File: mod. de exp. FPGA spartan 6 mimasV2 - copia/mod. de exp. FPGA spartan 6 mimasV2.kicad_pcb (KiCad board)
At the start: 2 copper layers, 111.5 x 57.8 mm, 46 parts, among them J1 locked, J2 locked, J3 locked, J4 locked, SW1 SW_DIP_x08, SW2 SW_Push, SW3 SW_Push, SW4 SW_Push, SW5 SW_Push, U1 CA56-12CGKWA

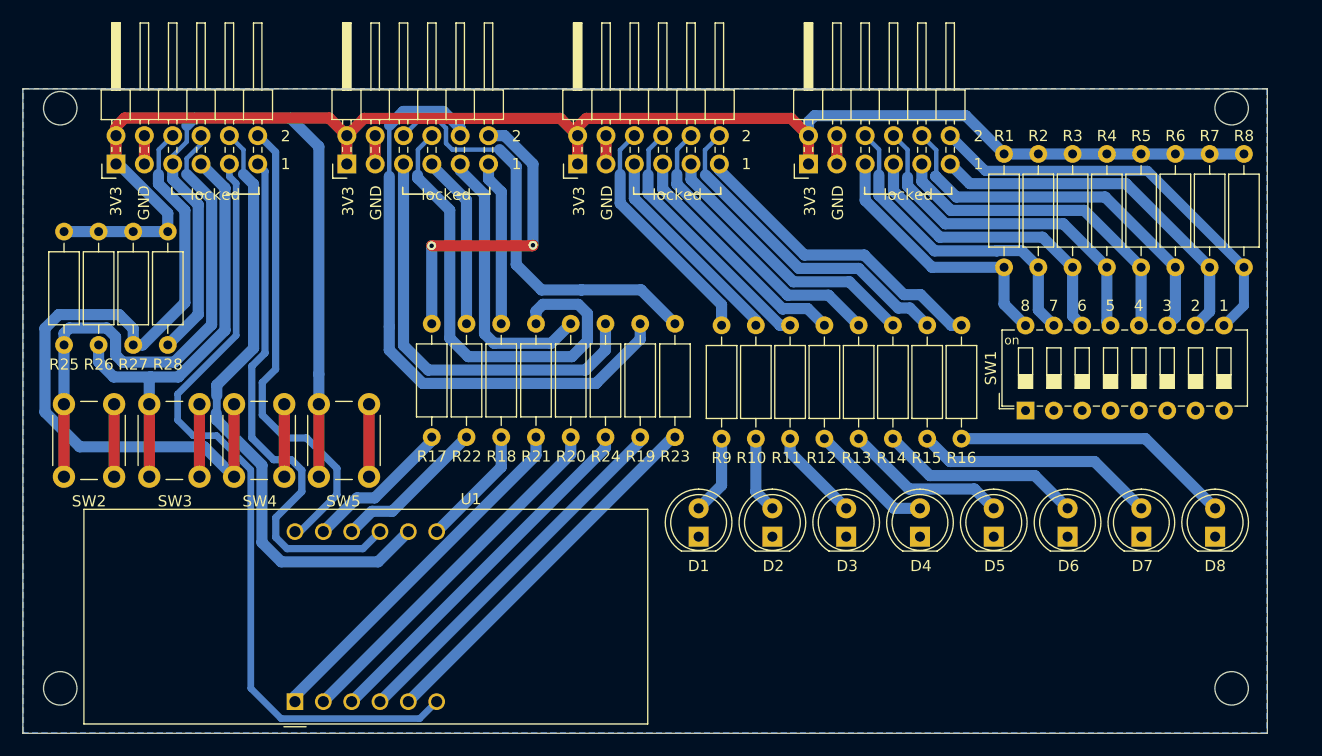
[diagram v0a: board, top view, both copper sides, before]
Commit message: absolutamente todo
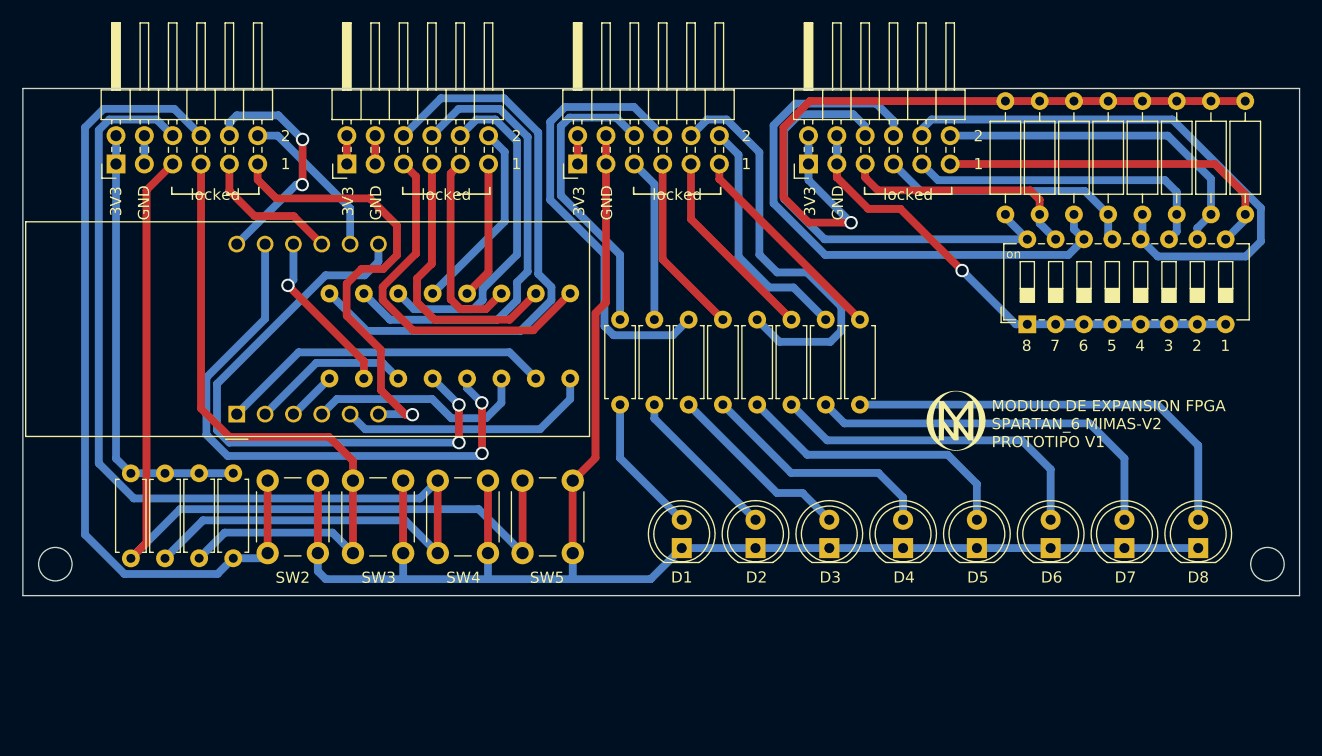
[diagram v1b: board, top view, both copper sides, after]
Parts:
- added G***: LOGO, wao:logo v2, F.Cu at (175.3, 123.0)
- R10, R11, R12, R13, R14, R15, R16, R25, R26, R27, R28, R9: footprint Resistor_THT:R_Axial_DIN0207_L6.3mm_D2.5mm_P10.16mm_Horizontal -> Resistor_THT:R_Axial_DIN0207_L6.3mm_D2.5mm_P7.62mm_Horizontal
- R17, R18, R19, R20, R21, R22, R23, R24: footprint Resistor_THT:R_Axial_DIN0207_L6.3mm_D2.5mm_P10.16mm_Horizontal -> Resistor_THT:R_Axial_DIN0207_L6.3mm_D2.5mm_P7.62mm_Horizontal; moved to B.Cu
- moved R25 26.4 mm to (110.5, 127.7)
- moved U1 26.3 mm to (110.8, 122.4)
- moved R24 24.9 mm to (119.1, 111.6)
- moved R26 23.5 mm to (107.5, 127.7)
- moved R28 21.9 mm to (101.3, 127.7)
- moved R27 21.9 mm to (104.4, 127.7)
- moved SW2 19.5 mm to (118.1, 128.4)
- moved SW4 19.5 mm to (133.3, 128.4)
- moved SW3 19.5 mm to (125.7, 128.4)
- moved SW5 19.5 mm to (140.9, 128.4)
- moved R20 15.7 mm to (125.3, 111.6)
- moved R19 12.7 mm to (134.5, 111.6)
- moved R23 9.77 mm to (140.7, 111.6)
- moved R22 9.59 mm to (122.2, 111.6)
- moved R15 9.11 mm to (163.6, 114.0)
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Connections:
- D1 pad 1: GND -> GND2
- D2 pad 1: GND -> GND2
- D3 pad 1: GND -> GND2
- D4 pad 1: GND -> GND2
- D5 pad 1: GND -> GND2
- D6 pad 1: GND -> GND2
- D7 pad 1: GND -> GND2
- D8 pad 1: GND -> GND2
- J2 pad 1: +3V3 -> +3.3V
- J2 pad 2: +3V3 -> +3.3V
- J2 pad 3: GND -> GND1
- J2 pad 4: GND -> GND1
- J3 pad 1: +3V3 -> +3.3VA
- J3 pad 2: +3V3 -> +3.3VA
- J3 pad 3: GND -> GND2
- J3 pad 4: GND -> GND2
- J4 pad 1: +3V3 -> +3.3VADC
- J4 pad 2: +3V3 -> +3.3VADC
- J4 pad 3: GND -> GND3
- J4 pad 4: GND -> GND3
- R1 pad 1: +3V3 -> +3.3VADC
- R1 pad 2: /DIP_SWITCH/7P9 -> /DIP_SWITCH/8P9
- R17 pad 1: /DISPLAY/2P7 -> /DISPLAY/1P7
- R18 pad 1: /DISPLAY/1P7 -> /DISPLAY/2P7
- R19 pad 1: /DISPLAY/4P7 -> /DISPLAY/3P7
- R2 pad 1: +3V3 -> +3.3VADC
- R2 pad 2: /DIP_SWITCH/8P9 -> /DIP_SWITCH/7P9
- R20 pad 1: /DISPLAY/3P7 -> /DISPLAY/4P7
- R21 pad 1: /DISPLAY/6P7 -> /DISPLAY/5P7
- R22 pad 1: /DISPLAY/5P7 -> /DISPLAY/6P7
- R23 pad 1: /DISPLAY/8P7 -> /DISPLAY/7P7
- R24 pad 1: /DISPLAY/7P7 -> /DISPLAY/8P7
- R3 pad 1: +3V3 -> +3.3VADC
- R3 pad 2: /DIP_SWITCH/5P9 -> /DIP_SWITCH/6P9
- R4 pad 1: +3V3 -> +3.3VADC
- R4 pad 2: /DIP_SWITCH/6P9 -> /DIP_SWITCH/5P9
- R5 pad 1: +3V3 -> +3.3VADC
- R5 pad 2: /DIP_SWITCH/3P9 -> /DIP_SWITCH/4P9
- R6 pad 1: +3V3 -> +3.3VADC
- R6 pad 2: /DIP_SWITCH/4P9 -> /DIP_SWITCH/3P9
- R7 pad 1: +3V3 -> +3.3VADC
- R7 pad 2: /DIP_SWITCH/1P9 -> /DIP_SWITCH/2P9
- R8 pad 1: +3V3 -> +3.3VADC
- R8 pad 2: /DIP_SWITCH/2P9 -> /DIP_SWITCH/1P9
- SW1 pad 1: GND -> GND3
- SW1 pad 10: /DIP_SWITCH/1P9 -> /DIP_SWITCH/2P9
- SW1 pad 11: /DIP_SWITCH/4P9 -> /DIP_SWITCH/3P9
- SW1 pad 12: /DIP_SWITCH/3P9 -> /DIP_SWITCH/4P9
- SW1 pad 13: /DIP_SWITCH/6P9 -> /DIP_SWITCH/5P9
- SW1 pad 14: /DIP_SWITCH/5P9 -> /DIP_SWITCH/6P9
- SW1 pad 15: /DIP_SWITCH/8P9 -> /DIP_SWITCH/7P9
- SW1 pad 16: /DIP_SWITCH/7P9 -> /DIP_SWITCH/8P9
- SW1 pad 2: GND -> GND3
- SW1 pad 3: GND -> GND3
- SW1 pad 4: GND -> GND3
- SW1 pad 5: GND -> GND3
- SW1 pad 6: GND -> GND3
- SW1 pad 7: GND -> GND3
- SW1 pad 8: GND -> GND3
- SW1 pad 9: /DIP_SWITCH/2P9 -> /DIP_SWITCH/1P9
- SW2 pad 1: GND -> GND2
- SW3 pad 1: GND -> GND2
- SW4 pad 1: GND -> GND2
- SW5 pad 1: GND -> GND2
- U1 pad 12: /DISPLAY/2P6 -> /DISPLAY/4P6
- U1 pad 6: /DISPLAY/3P6 -> /DISPLAY/1P6
- U1 pad 8: /DISPLAY/4P6 -> /DISPLAY/2P6
- U1 pad 9: /DISPLAY/1P6 -> /DISPLAY/3P6
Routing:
- net GND2: track 0.00 -> 147.3 mm
- net +3V3: track 136.4 -> 40.0 mm
- net +3.3VADC: track 0.00 -> 65.0 mm, vias 0 -> 1
- net /DISPLAY/3P6: track 71.8 -> 12.7 mm
- net GND3: track 0.00 -> 44.1 mm, vias 0 -> 1
- net Net-(U1-b): track 10.9 -> 53.6 mm, vias 0 -> 2
- net Net-(U1-a): track 13.4 -> 52.1 mm, vias 0 -> 2
- net /PIN_HEADER_8X4/8P6: track 66.4 -> 103.4 mm
- net /DISPLAY/4P6: track 55.4 -> 21.0 mm, vias 0 -> 2
- net GND: track 36.2 -> 2.54 mm
- net Net-(U1-DPX): track 33.1 -> 4.55 mm
- net /DISPLAY/2P6: track 42.4 -> 14.2 mm
- net /PIN_HEADER_8X4/6P6: track 48.3 -> 73.7 mm
- net /DISPLAY/4P7: track 55.1 -> 30.5 mm
- net /DIP_SWITCH/6P9: track 31.3 -> 53.4 mm
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- removed copper zone on B.Cu, net GND
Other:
- board size 111.5 x 57.8 mm -> 114.4 x 45.5 mm
- board text added: "MODULO DE EXPANSION FPGA SPARTAN_6 MIMAS-V2 PROTOTIPO V1"
